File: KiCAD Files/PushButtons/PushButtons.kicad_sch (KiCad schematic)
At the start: 8 parts, among them J1 Conn_01x04_Pin, SW1 SW_Push, SW2 SW_Push, SW3 SW_Push

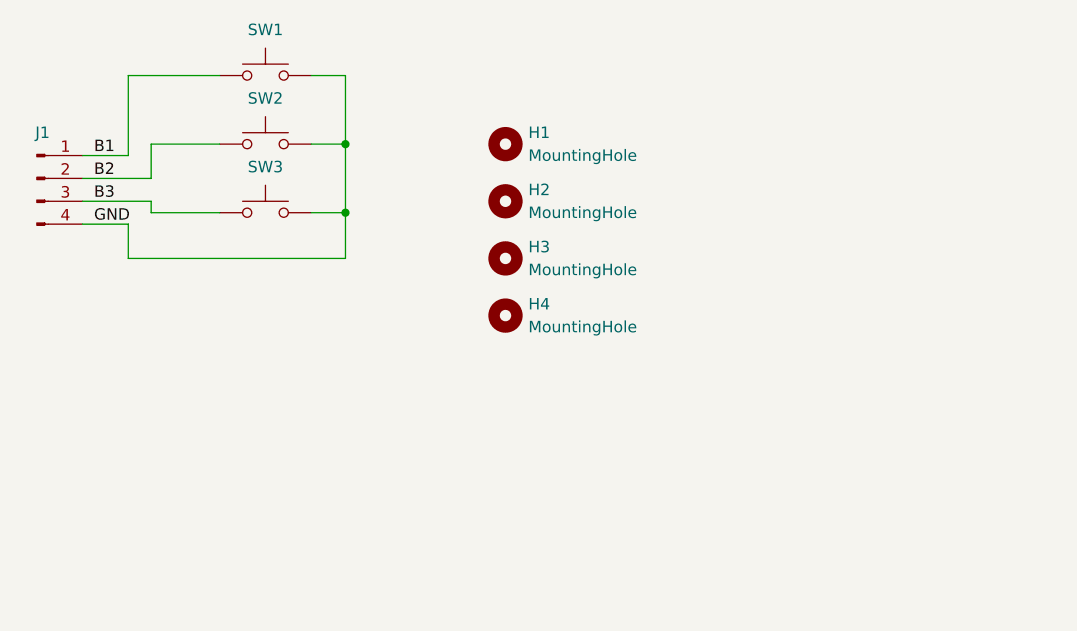
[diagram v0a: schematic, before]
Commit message: update
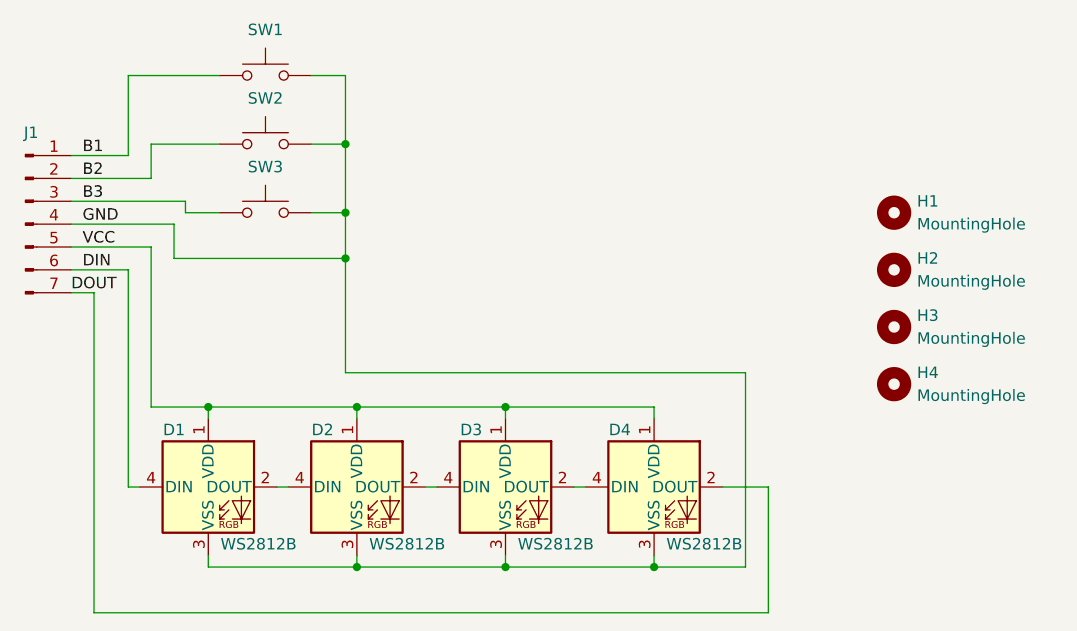
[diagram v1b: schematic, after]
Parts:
- removed J1: Conn_01x04_Pin, Connector_PinHeader_2.54mm:PinHeader_1x04_P2.54mm_Horizontal, symbol Connector:Conn_01x04_Pin
- added D1, D2, D3, D4: WS2812B, LED_SMD:LED_WS2812B_PLCC4_5.0x5.0mm_P3.2mm, symbol LED:WS2812B
- added J1: Conn_01x07_Pin, symbol Connector:Conn_01x07_Pin
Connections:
- net B1: now also J1.1 (Pin_1)
- net B2: now also J1.2 (Pin_2)
- net B3: now also J1.3 (Pin_3)
- net GND: now also D1.3 (VSS), D2.3 (VSS), D3.3 (VSS), D4.3 (VSS), J1.4 (Pin_4)
- new net: D3.2 (DOUT), D4.4 (DIN)
- new net: D2.2 (DOUT), D3.4 (DIN)
- new net: D1.2 (DOUT), D2.4 (DIN)
- new net DIN: D1.4 (DIN), J1.6 (Pin_6)
- new net DOUT: D4.2 (DOUT), J1.7 (Pin_7)
- new net VCC: D1.1 (VDD), D2.1 (VDD), D3.1 (VDD), D4.1 (VDD), J1.5 (Pin_5)
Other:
- moved on the sheet: H1, H2, H3, H4

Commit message: update
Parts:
- J1: footprint (none) -> Connector_PinHeader_2.54mm:PinHeader_1x07_P2.54mm_Horizontal
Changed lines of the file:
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@@
 			)
 		)
-		(property "Footprint" ""
+		(property "Footprint" "Connector_PinHeader_2.54mm:PinHeader_1x07_P2.54mm_Horizontal"
 			(at 106.68 100.33 0)
 			(effects
